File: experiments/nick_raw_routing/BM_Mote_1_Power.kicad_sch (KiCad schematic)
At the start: 26 parts, among them U10 LMR51430YDDCR, U5 LMR51430YDDCR, U6 TPS62840YBGR

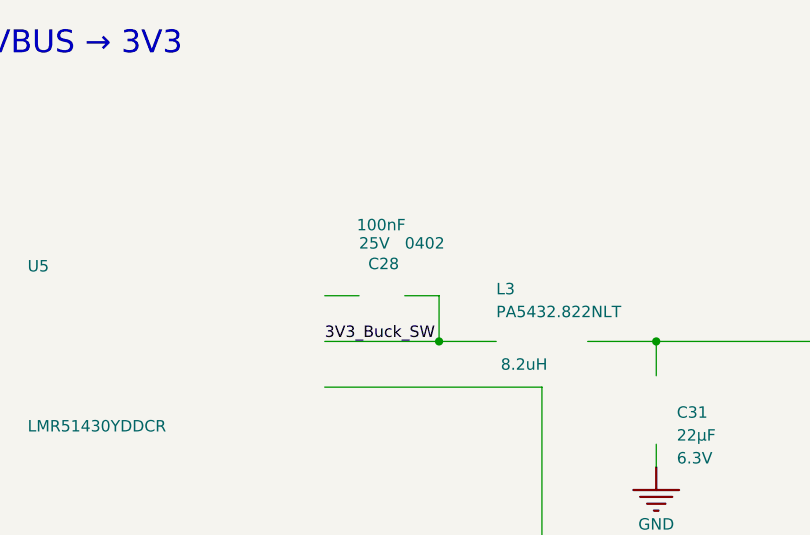
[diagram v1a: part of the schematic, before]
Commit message: Fix import connectivity
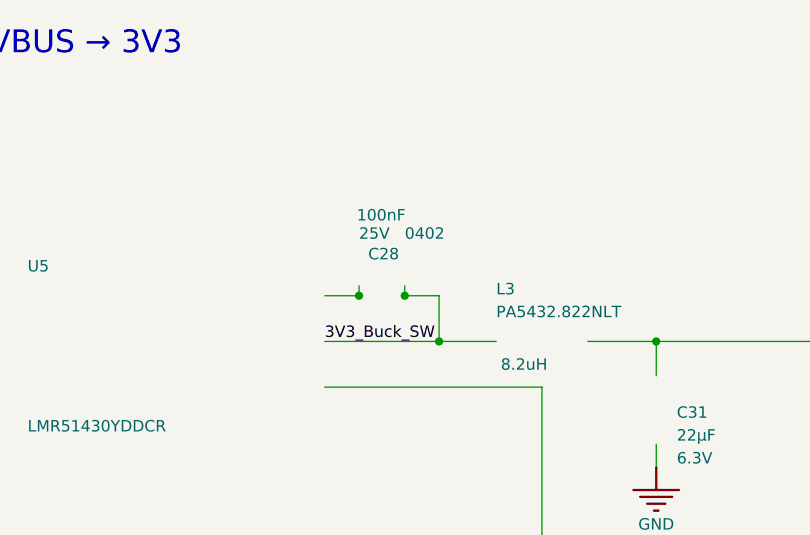
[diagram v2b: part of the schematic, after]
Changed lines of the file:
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@@
 	)
 	(junction
+		(at 177.8 78.5622)
+		(diameter 0)
+		(color 0 0 0 0)
+	)
+	(junction
 		(at 95.25 215.7222)
 		(diameter 0)
@@
 	)
 	(junction
+		(at 172.72 78.5622)
+		(diameter 0)
+		(color 0 0 0 0)
+	)
+	(junction
 		(at 74.93 239.8522)
 		(diameter 0)
@@
 	(wire
 		(pts
+			(xy 177.8 78.5622) (xy 177.8 78.74)
+		)
+		(stroke
+			(width 0)
+			(type default)
+		)
+	)
+	(wire
+		(pts
 			(xy 181.61 220.8022) (xy 187.96 220.8022)
 		)
@@
 	(wire
 		(pts
+			(xy 172.72 77.47) (xy 172.72 78.5622)
+		)
+		(stroke
+			(width 0)
+			(type default)
+		)
+	)
+	(wire
+		(pts
 			(xy 205.74 97.6122) (xy 205.74 95.0722)
 		)
@@
 	(wire
 		(pts
+			(xy 172.72 78.5622) (xy 172.72 78.74)
+		)
+		(stroke
+			(width 0)
+			(type default)
+		)
+	)
+	(wire
+		(pts
+			(xy 177.8 77.47) (xy 177.8 78.5622)
+		)
+		(stroke
+			(width 0)
+			(type default)
+		)
+	)
+	(wire
+		(pts
 			(xy 128.27 225.8822) (xy 125.73 225.8822)
 		)
@@
 	(symbol
 		(lib_id "BM_Mote_000639-AB-altium-import:POWER_3_b4654b650e69147ec39a6b967a45e02_Altium Content Vault")
-		(at 177.8 78.5622 0)
+		(at 177.8 77.47 0)
 		(unit 0)
 		(body_style 1)
@@
 		(dnp no)
 		(property "Reference" "C28"
-			(at 173.736 75.7682 0)
+			(at 173.736 74.676 0)
 			(show_name no)
 			(do_not_autoplace no)
@@
 		)
 		(property "Value" "CL05A104KA5NNNC"
-			(at 172.212 75.7682 0)
+			(at 172.212 74.676 0)
 			(hide yes)
 			(show_name no)
@@
 		)
 		(property "Footprint" "Vault:FP-CL278-IPC_C"
-			(at 177.8 78.5622 0)
+			(at 177.8 77.47 0)
 			(hide yes)
 			(show_name no)
@@
 		)
 		(property "Datasheet" ""
-			(at 177.8 78.5622 0)
+			(at 177.8 77.47 0)
 			(hide yes)
 			(show_name no)
@@
 		)
 		(property "Description" "Cap Ceramic 100nF 25V X5R ±10% SMD 0402 +85°C Paper T/R"
-			(at 177.8 78.5622 0)
+			(at 177.8 77.47 0)
 			(hide yes)
 			(show_name no)
@@
 		)
 		(property "PACKAGE QUANTITY" "1"
-			(at 172.212 75.7682 0)
+			(at 172.212 74.676 0)
 			(hide yes)
 			(show_name no)
@@
 		)
 		(property "HEIGHT" "0.5mm"
-			(at 172.212 75.7682 0)
+			(at 172.212 74.676 0)
 			(hide yes)
 			(show_name no)
@@
 		)
 		(property "CASE CODE (METRIC)" "1005"
-			(at 172.212 75.7682 0)
+			(at 172.212 74.676 0)
 			(hide yes)
 			(show_name no)
@@
 		)
 		(property "THICKNESS" "0.022inch"
-			(at 172.212 75.7682 0)
+			(at 172.212 74.676 0)
 			(hide yes)
 			(show_name no)
@@
 		)
 		(property "MOUNT" "Surface Mount"
-			(at 172.212 75.7682 0)
+			(at 172.212 74.676 0)
 			(hide yes)
 			(show_name no)
@@
 		)
 		(property "LEAD FREE" "Lead Free"
-			(at 172.212 75.7682 0)
+			(at 172.212 74.676 0)
 			(hide yes)
 			(show_name no)
@@
 		)
 		(property "CASE CODE (IMPERIAL)" "0402"
-			(at 177.8 73.4822 0)
+			(at 177.8 72.39 0)
 			(show_name no)
 			(do_not_autoplace no)
@@
 		)
 		(property "PACKAGING" "Tape and Reel"
-			(at 172.212 75.7682 0)
+			(at 172.212 74.676 0)
 			(hide yes)
 			(show_name no)
@@
 		)
 		(property "DEPTH" "0.5mm"
-			(at 172.212 75.7682 0)
+			(at 172.212 74.676 0)
 			(hide yes)
 			(show_name no)
@@
 		)
 		(property "VOLTAGE" "25V"
-			(at 172.72 73.4822 0)
+			(at 172.72 72.39 0)
 			(show_name no)
 			(do_not_autoplace no)
@@
 		)
 		(property "MIN OPERATING TEMPERATURE" "-55°C"
-			(at 172.212 75.7682 0)
+			(at 172.212 74.676 0)
 			(hide yes)
 			(show_name no)
@@
 		)
 		(property "VOLTAGE RATING" "25V"
-			(at 172.212 75.7682 0)
+			(at 172.212 74.676 0)
 			(hide yes)
 			(show_name no)
@@
 		)
 		(property "DIELECTRIC" "X5R"
-			(at 172.212 75.7682 0)
+			(at 172.212 74.676 0)
 			(hide yes)
 			(show_name no)
@@
 		)
 		(property "CASE/PACKAGE" "0402"
-			(at 172.212 75.7682 0)
+			(at 172.212 74.676 0)
 			(hide yes)
 			(show_name no)
@@
 		)
 		(property "TOLERANCE" "10%"
-			(at 172.212 75.7682 0)
+			(at 172.212 74.676 0)
 			(hide yes)
 			(show_name no)
@@
 		)
 		(property "WIDTH" "0.02inch"
-			(at 172.212 75.7682 0)
+			(at 172.212 74.676 0)
 			(hide yes)
 			(show_name no)
@@
 		)
 		(property "MAX OPERATING TEMPERATURE" "85°C"
-			(at 172.212 75.7682 0)
+			(at 172.212 74.676 0)
 			(hide yes)
 			(show_name no)
@@
 		)
 		(property "CAPACITANCE" "100nF"
-			(at 172.466 71.4502 0)
+			(at 172.466 70.358 0)
 			(show_name no)
 			(do_not_autoplace no)
@@
 		)
 		(property "LENGTH" "1mm"
-			(at 172.212 75.7682 0)
+			(at 172.212 74.676 0)
 			(hide yes)
 			(show_name no)
@@
 		)
 		(property "RADIATION HARDENING" "No"
-			(at 172.212 75.7682 0)
+			(at 172.212 74.676 0)
 			(hide yes)
 			(show_name no)
@@
 		)
 		(property "VOLTAGE RATING (DC)" "25V"
-			(at 172.212 75.7682 0)
+			(at 172.212 74.676 0)
 			(hide yes)
 			(show_name no)
@@
 		)
 		(property "SHEET" "ADIN2111"
-			(at 172.212 75.7682 0)
+			(at 172.212 74.676 0)
 			(hide yes)
 			(show_name no)
@@
 		)
 		(property "PLANNED MPN" "CL05A104KA5NNNC"
-			(at 177.8 78.5622 0)
+			(at 177.8 77.47 0)
 			(hide yes)
 			(show_name no)
@@
 		)
 		(property "PLANNED MFR" "Samsung"
-			(at 177.8 78.5622 0)
+			(at 177.8 77.47 0)
 			(hide yes)
 			(show_name no)
@@
 		)
 		(property "PLANNED LCSC" "C100072"
-			(at 177.8 78.5622 0)
+			(at 177.8 77.47 0)
 			(hide yes)
 			(show_name no)
@@
 		)
 		(property "PLANNED NOTE" "As specified; in LCSC stock (checked 2026-10-06)"
-			(at 177.8 78.5622 0)
+			(at 177.8 77.47 0)
 			(hide yes)
 			(show_name no)
@@
 		)
 		(property "MANUFACTURER" "Samsung"
-			(at 177.8 78.5622 0)
+			(at 177.8 77.47 0)
 			(hide yes)
 			(show_name no)
